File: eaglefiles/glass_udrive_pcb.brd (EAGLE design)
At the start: 14.9 x 20 mm, 31 parts

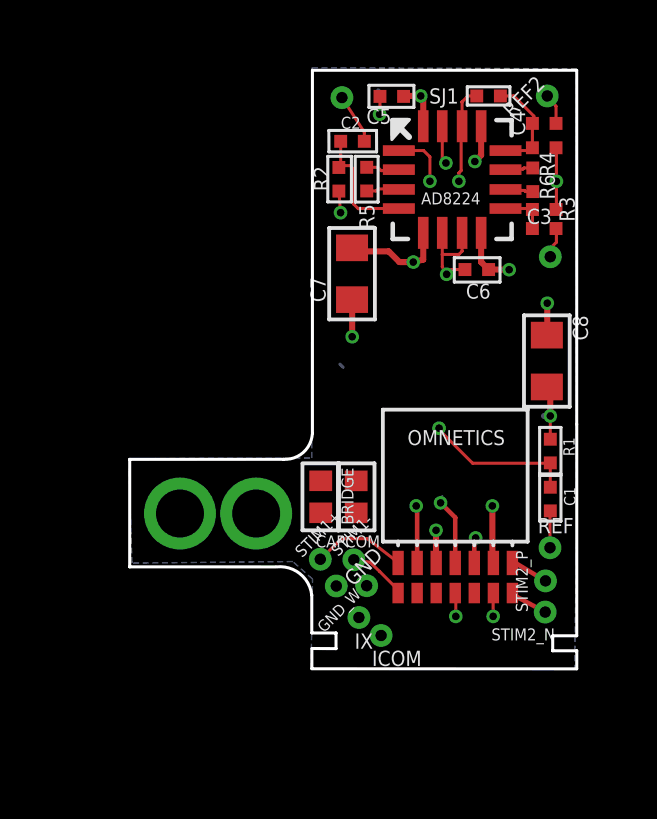
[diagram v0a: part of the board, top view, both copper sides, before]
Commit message: simple routing finish-up and silk-screen stuff.
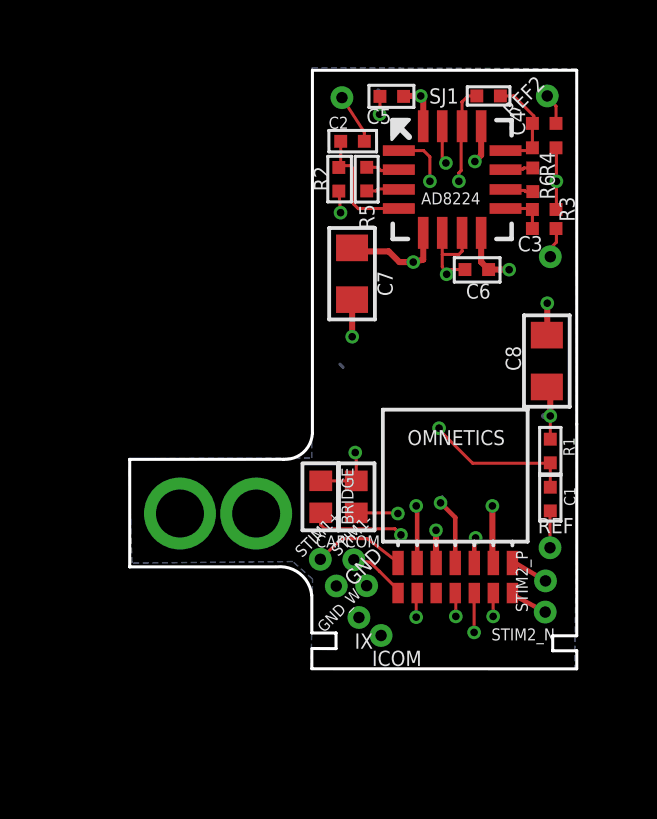
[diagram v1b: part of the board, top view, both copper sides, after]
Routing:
- net GLASS: track 1.68 -> 16.3 mm, vias 0 -> 1
- net BRG_BAL: track 0.00 -> 10.2 mm, vias 0 -> 2
- net CAP_COM: track 0.00 -> 6.04 mm, vias 0 -> 2
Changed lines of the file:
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@@
 </element>
 <element name="C2" library="GFL" package="0201" value="6800pF" x="8.1388" y="17.6896" smashed="yes" rot="R180">
-<attribute name="NAME" x="7.7488" y="18.1088" size="0.4" layer="25"/>
+<attribute name="NAME" x="7.3424" y="18.1088" size="0.4" layer="25"/>
 <attribute name="VALUE" x="8.7738" y="19.5946" size="1.27" layer="27" rot="R180"/>
 </element>
@@
 </element>
 <element name="C7" library="GFL" package="0603" value="10uF" x="8.1232" y="13.2764" smashed="yes" rot="R90">
-<attribute name="NAME" x="6.7358" y="13.165" size="0.508" layer="25" font="vector" rot="R270"/>
+<attribute name="NAME" x="8.971" y="13.3682" size="0.508" layer="25" font="vector" rot="R270"/>
 <attribute name="VALUE" x="9.698" y="12.0826" size="1.016" layer="27" font="vector" rot="R90"/>
 </element>
 <element name="C8" library="GFL" package="0603" value="10uF" x="14.6164" y="10.3656" smashed="yes" rot="R90">
-<attribute name="NAME" x="15.988" y="11.0514" size="0.508" layer="25" font="vector" rot="R90"/>
+<attribute name="NAME" x="13.7528" y="10.0354" size="0.508" layer="25" font="vector" rot="R90"/>
 <attribute name="VALUE" x="16.1912" y="9.1718" size="1.016" layer="27" font="vector" rot="R90"/>
 </element>
@@
 </element>
 <element name="C3" library="GFL" package="0201" value="6800pF" x="14.5288" y="14.7828" smashed="yes" rot="R180">
-<attribute name="NAME" x="14.7828" y="15.4432" size="0.508" layer="25" font="vector" rot="R180"/>
+<attribute name="NAME" x="14.478" y="14.5288" size="0.508" layer="25" font="vector" rot="R180"/>
 <attribute name="VALUE" x="15.7226" y="16.3576" size="1.016" layer="27" font="vector" rot="R180"/>
 </element>
@@
 <contactref element="OMNETICS" pad="V"/>
 <contactref element="CAPCOM" pad="2"/>
-<wire x1="8.262" y1="5.30489375" x2="10.2934" y2="2.6319" width="0" layer="19" extent="1-1"/>
+<wire x1="8.262" y1="5.30489375" x2="9.63030625" y2="5.30489375" width="0.1016" layer="1"/>
+<wire x1="9.63030625" y1="5.30489375" x2="9.652" y2="5.2832" width="0.1016" layer="1"/>
+<via x="9.652" y="5.2832" extent="1-16" drill="0.254"/>
+<wire x1="9.652" y1="5.2832" x2="9.8552" y2="5.2832" width="0.1016" layer="15"/>
+<wire x1="9.8552" y1="5.2832" x2="10.2616" y2="4.8768" width="0.1016" layer="15"/>
+<wire x1="10.2616" y1="4.8768" x2="10.2616" y2="1.8288" width="0.1016" layer="15"/>
+<via x="10.2616" y="1.8288" extent="1-16" drill="0.254"/>
+<wire x1="10.2616" y1="1.8288" x2="10.2616" y2="2.6001" width="0.1016" layer="1"/>
+<wire x1="10.2616" y1="2.6001" x2="10.2934" y2="2.6319" width="0.1016" layer="1"/>
 </signal>
 <signal name="STIM1_P">
@@
 <contactref element="OMNETICS" pad="B"/>
 <contactref element="BRIDGE" pad="2"/>
-<wire x1="7.079678125" y1="5.30709375" x2="12.1984" y2="2.6319" width="0" layer="19" extent="1-1"/>
+<wire x1="7.079678125" y1="5.30709375" x2="7.079678125" y2="4.909121875" width="0.1016" layer="1"/>
+<wire x1="7.079678125" y1="4.909121875" x2="7.2136" y2="4.7752" width="0.1016" layer="1"/>
+<wire x1="7.2136" y1="4.7752" x2="9.5504" y2="4.7752" width="0.1016" layer="1"/>
+<wire x1="9.5504" y1="4.7752" x2="9.7536" y2="4.572" width="0.1016" layer="1"/>
+<via x="9.7536" y="4.572" extent="1-16" drill="0.254"/>
+<wire x1="9.7536" y1="4.572" x2="9.7536" y2="1.524" width="0.1016" layer="15"/>
+<wire x1="9.7536" y1="1.524" x2="10.16" y2="1.2192" width="0.1016" layer="15"/>
+<wire x1="10.16" y1="1.2192" x2="12.0904" y2="1.2192" width="0.1016" layer="15"/>
+<wire x1="12.0904" y1="1.2192" x2="12.192" y2="1.3208" width="0.1016" layer="15"/>
+<via x="12.192" y="1.3208" extent="1-16" drill="0.254"/>
+<wire x1="12.192" y1="1.3208" x2="12.192" y2="2.6255" width="0.1016" layer="1"/>
+<wire x1="12.192" y1="2.6255" x2="12.1984" y2="2.6319" width="0.1016" layer="1"/>
 </signal>
 <signal name="I_COM">
@@
 <wire x1="8.5325" y1="17.6896" x2="8.5325" y2="17.9973" width="0.1016" layer="1"/>
 <wire x1="8.5325" y1="17.9973" x2="7.7866" y2="19.1464" width="0.1016" layer="1"/>
-<wire x1="8.262" y1="6.37169375" x2="8.5325" y2="17.6896" width="0" layer="19" extent="1-1"/>
-<wire x1="7.079678125" y1="6.37389375" x2="8.262" y2="6.37169375" width="0" layer="19" extent="1-1"/>
+<wire x1="7.079678125" y1="6.37389375" x2="7.081878125" y2="6.37169375" width="0.1016" layer="1"/>
+<wire x1="7.081878125" y1="6.37169375" x2="8.262" y2="6.37169375" width="0.1016" layer="1"/>
+<wire x1="8.262" y1="6.37169375" x2="8.262" y2="7.2828" width="0.1016" layer="1"/>
+<wire x1="8.262" y1="7.2828" x2="8.2296" y2="7.3152" width="0.1016" layer="1"/>
+<via x="8.2296" y="7.3152" extent="1-16" drill="0.254"/>
+<wire x1="8.2296" y1="7.3152" x2="8.2296" y2="10.4648" width="0.1016" layer="15"/>
+<wire x1="8.2296" y1="10.4648" x2="8.7376" y2="10.9728" width="0.1016" layer="15"/>
+<wire x1="8.7376" y1="10.9728" x2="8.7376" y2="18.1954" width="0.1016" layer="15"/>
+<wire x1="8.7376" y1="18.1954" x2="7.7866" y2="19.1464" width="0.1016" layer="15"/>
 </signal>
 <signal name="GLASS_OUT">
